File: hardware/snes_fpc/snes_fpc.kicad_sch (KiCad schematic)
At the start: 12 parts, among them J2 Connector_Generic:Conn_02x16_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, J4 Conn_01x02_Pin, U1 74HC175, U2 CD4078B, U3 74AHC1G08, U4 74AHC1G08

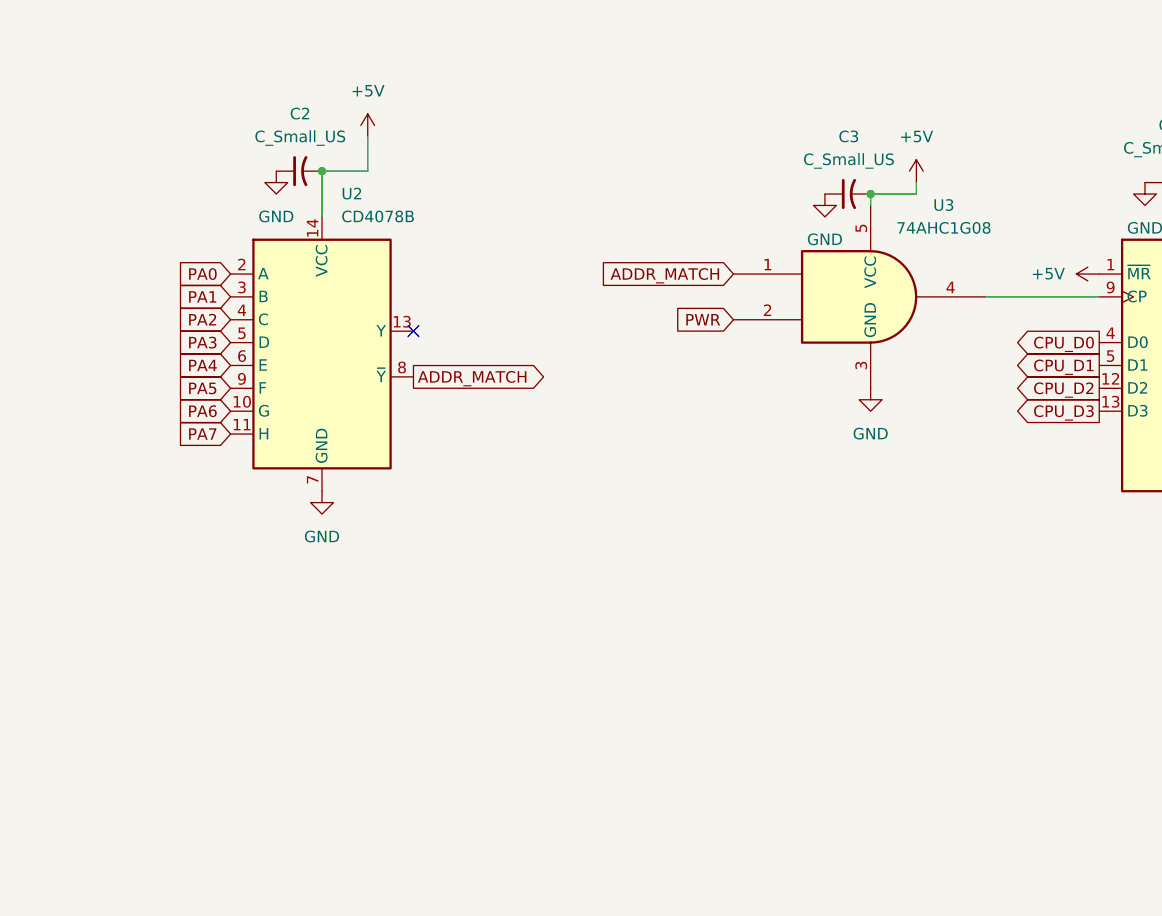
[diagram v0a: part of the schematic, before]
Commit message: update fpc
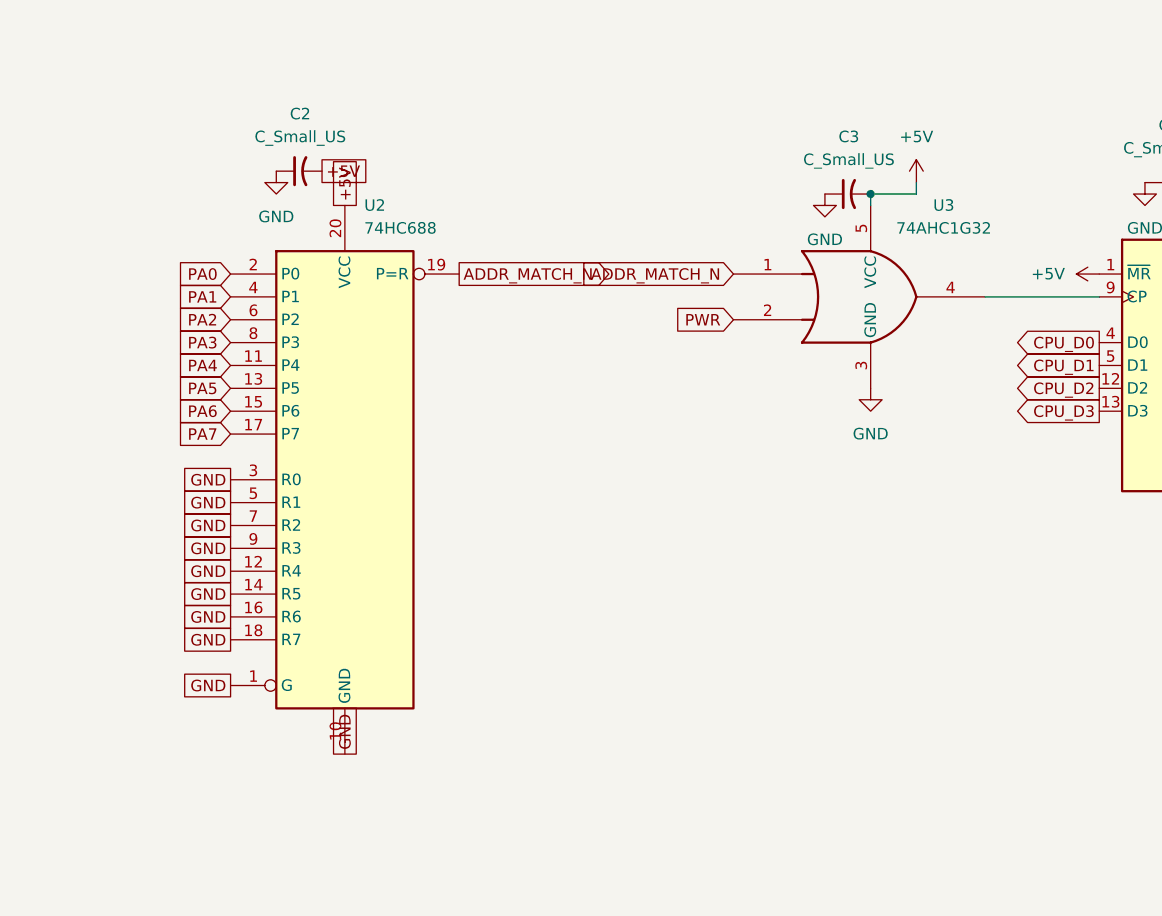
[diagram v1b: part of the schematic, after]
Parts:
- U2: value CD4078B -> 74HC688; footprint Package_SO:TSSOP-14_4.4x5mm_P0.65mm -> Package_SO:TSSOP-20_4.4x6.5mm_P0.65mm; symbol Snes:74HC4078 -> Snes:74HC688; JLCPCB Part # C2682016 -> C132045; LCSC C2682016 -> C132045; LCSC Part C2682016 -> C132045; LCSC Part # C2682016 -> C132045; LCSC Part Name CD4078BPWR -> SN74HC688PWR; MPN CD4078BPWR -> SN74HC688PWR; Manufacturer Part CD4078BPWR -> SN74HC688PWR; Sourcing Note Pin-compatible TSSOP-14 LCSC/JLC 8-input OR/NOR candidate; 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 -> Fast HC TSSOP-20 comparator used as PA0-PA7 zero detector; 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; Supplier Part C2682016 -> C132045; Supplier URL https://www.lcsc.com/product-detail/C2682016.html -> https://www.lcsc.com/product-detail/C132045.html
- U3: value 74AHC1G08 -> 74AHC1G32; symbol 74xGxx:74AHC1G08 -> Snes:74AHC1G32; JLCPCB Part # C7467 -> C7470; LCSC C7467 -> C7470; LCSC Part C7467 -> C7470; LCSC Part # C7467 -> C7470; LCSC Part Name SN74AHC1G08DBVR -> SN74AHC1G32DBVR; MPN SN74AHC1G08DBVR -> SN74AHC1G32DBVR; Manufacturer Part SN74AHC1G08DBVR -> SN74AHC1G32DBVR; Sourcing Note (none) -> OR gate used with active-low SN74HC688 equality output and 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; Supplier Part C7467 -> C7470; Supplier URL https://www.lcsc.com/product-detail/Gates_Texas-Instruments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 -> https://www.lcsc.com/product-detail/C7470.html
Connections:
- net +5V: now also U2.20 (VCC); no longer U2.14 (VCC)
- net GND: now also U2.1 (G), U2.10 (GND), U2.12 (R4), U2.14 (R5), U2.16 (R6), U2.18 (R7), U2.3 (R0), U2.5 (R1), U2.9 (R3)
- net PA1: now also U2.4 (P1); no longer U2.3 (B)
- net PA2: now also U2.6 (P2); no longer U2.4 (C)
- net PA3: now also U2.8 (P3); no longer U2.5 (D)
- net PA4: now also U2.11 (P4); no longer U2.6 (E)
- net PA5: now also U2.13 (P5); no longer U2.9 (F)
- net PA6: now also U2.15 (P6); no longer U2.10 (G)
- net PA7: now also U2.17 (P7); no longer U2.11 (H)
- net ADDR_MATCH renamed ADDR_MATCH_N
- net ADDR_MATCH_N: now also U2.19 (P=R); no longer U2.8 (~{Y})
- no-connect marks 8 -> 7
